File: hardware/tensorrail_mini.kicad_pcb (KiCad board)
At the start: 2 copper layers, 100 x 70 mm, 62 parts, among them J1 USB-C_PWR, J2 JTAG, J3 EXPANSION, SW1 RESET, SW2 BOOT, U1 TPS62130_3V3, U2 TPS62130_1V2, U3 INA219, U4 W25Q128, U5 50MHz

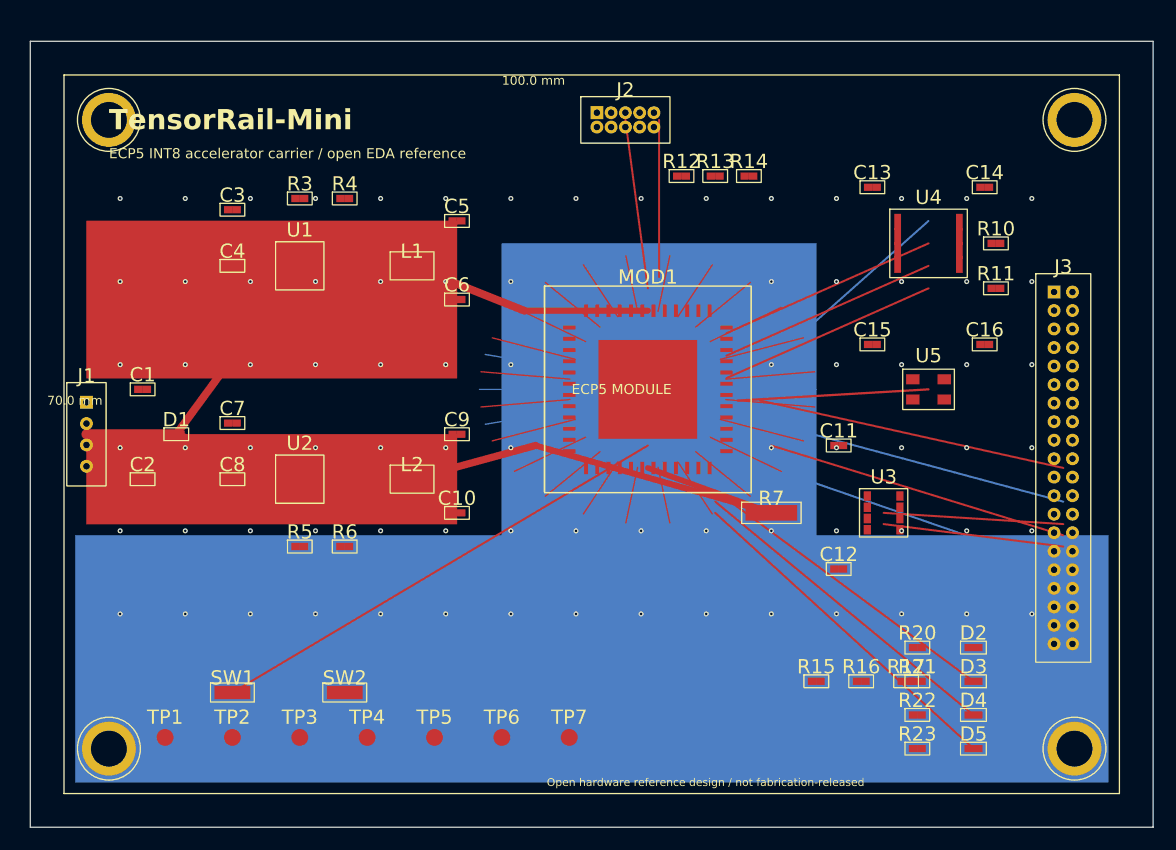
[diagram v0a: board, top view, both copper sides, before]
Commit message: Update TensorRail PCB artifact
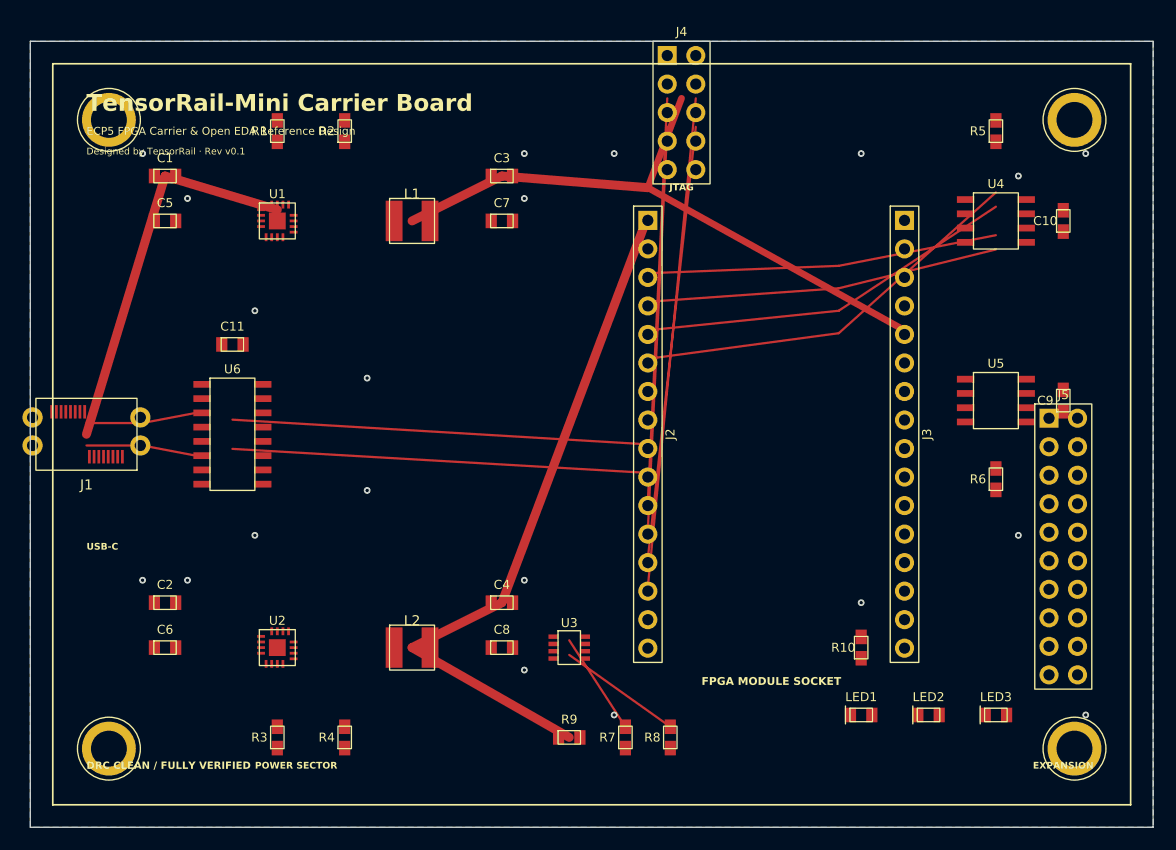
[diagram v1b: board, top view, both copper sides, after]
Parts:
- removed C12: 10n, Discrete_SMD:C12
- removed C13: 100n, Discrete_SMD:C13
- removed C14: 10n, Discrete_SMD:C14
- removed C15: 100n, Discrete_SMD:C15
- removed C16: 10n, Discrete_SMD:C16
- removed D1: PMEG, Discrete_SMD:D1
- removed D2: LED, Discrete_SMD:D2
- removed D3: LED, Discrete_SMD:D3
- removed D4: LED, Discrete_SMD:D4
- removed D5: LED, Discrete_SMD:D5
- removed MOD1: OrangeCrab_85F, Module:ECP5_Feather_Module_Socket
- removed R11: 10k, Discrete_SMD:R11
- removed R12: 100R, Discrete_SMD:R12
- removed R13: 100R, Discrete_SMD:R13
- removed R14: 100R, Discrete_SMD:R14
- removed R15: 4k7, Discrete_SMD:R15
- removed R16: 4k7, Discrete_SMD:R16
- removed R17: 4k7, Discrete_SMD:R17
- removed R20: 330R, Discrete_SMD:R20
- removed R21: 330R, Discrete_SMD:R21
- removed R22: 330R, Discrete_SMD:R22
- removed R23: 330R, Discrete_SMD:R23
- removed SW1: RESET, Discrete_SMD:SW1
- removed SW2: BOOT, Discrete_SMD:SW2
- removed TP1: +5V, TestPoint:TestPoint_Pad_D1.5mm
- removed TP2: +3V3, TestPoint:TestPoint_Pad_D1.5mm
- removed TP3: +1V2, TestPoint:TestPoint_Pad_D1.5mm
- removed TP4: GND, TestPoint:TestPoint_Pad_D1.5mm
- removed TP5: SCL, TestPoint:TestPoint_Pad_D1.5mm
- removed TP6: SDA, TestPoint:TestPoint_Pad_D1.5mm
- removed TP7: CLK_50M, TestPoint:TestPoint_Pad_D1.5mm
- added J4: JTAG, Connector_PinHeader_2.54mm:PinHeader_2x05_P2.54mm_Vertical, F.Cu at (58.0, 6.35)
- added J5: EXPANSION, Connector_PinHeader_2.54mm:PinHeader_2x10_P2.54mm_Vertical, F.Cu at (92.0, 45.0)
- added LED1: Green, LED_SMD:LED_0805_2012Metric, F.Cu at (74.0, 60.0)
- added LED2: Blue, LED_SMD:LED_0805_2012Metric, F.Cu at (80.0, 60.0)
- added LED3: Red, LED_SMD:LED_0805_2012Metric, F.Cu at (86.0, 60.0)
- added R1: 464k, Resistor_SMD:R_0805_2012Metric, F.Cu at (22.0, 8.00)
- added R2: 100k, Resistor_SMD:R_0805_2012Metric, F.Cu at (28.0, 8.00)
- added R8: 10k, Resistor_SMD:R_0805_2012Metric, F.Cu at (57.0, 62.0)
- added R9: 0.1, Resistor_SMD:R_0805_2012Metric, F.Cu at (48.0, 62.0)
- added U6: CH340C, Package_SO:SOIC-16_3.9x9.9mm_P1.27mm, F.Cu at (18.0, 35.0)
- C1: value 100n -> 10u; footprint Discrete_SMD:C1 -> Capacitor_SMD:C_0805_2012Metric
- C10: footprint Discrete_SMD:C10 -> Capacitor_SMD:C_0805_2012Metric
- C11: value 100n -> 22u; footprint Discrete_SMD:C11 -> Capacitor_SMD:C_0805_2012Metric
- C2: value 100n -> 10u; footprint Discrete_SMD:C2 -> Capacitor_SMD:C_0805_2012Metric
- C3: footprint Discrete_SMD:C3 -> Capacitor_SMD:C_0805_2012Metric
- C4: value 100n -> 10u; footprint Discrete_SMD:C4 -> Capacitor_SMD:C_0805_2012Metric
- C5: value 100u -> 100n; footprint Discrete_SMD:C5 -> Capacitor_SMD:C_0805_2012Metric
- C6: footprint Discrete_SMD:C6 -> Capacitor_SMD:C_0805_2012Metric
- C7: value 10u -> 100n; footprint Discrete_SMD:C7 -> Capacitor_SMD:C_0805_2012Metric
- C8: footprint Discrete_SMD:C8 -> Capacitor_SMD:C_0805_2012Metric
- C9: value 100u -> 100n; footprint Discrete_SMD:C9 -> Capacitor_SMD:C_0805_2012Metric
- J1: value USB-C_PWR -> USB-C; footprint Connector_Generic:1x4_Header -> Connector_USB:USB_C_Receptacle_GCT_USB4135
- J2: value JTAG -> Feather Left; footprint Connector_Generic:5x2_Header -> Connector_PinHeader_2.54mm:PinHeader_1x16_P2.54mm_Vertical
- J3: value EXPANSION -> Feather Right; footprint Connector_Generic:2x20_Header -> Connector_PinHeader_2.54mm:PinHeader_1x16_P2.54mm_Vertical
- L1: footprint Discrete_SMD:L1 -> Inductor_SMD:L_Bourns-SRN4018
- L2: footprint Discrete_SMD:L2 -> Inductor_SMD:L_Bourns-SRN4018
- R10: value 10k -> 330; footprint Discrete_SMD:R10 -> Resistor_SMD:R_0805_2012Metric
- R3: value 464k -> 103k; footprint Discrete_SMD:R3 -> Resistor_SMD:R_0805_2012Metric
- R4: footprint Discrete_SMD:R4 -> Resistor_SMD:R_0805_2012Metric
- R5: value 103k -> 10k; footprint Discrete_SMD:R5 -> Resistor_SMD:R_0805_2012Metric
- R6: value 100k -> 10k; footprint Discrete_SMD:R6 -> Resistor_SMD:R_0805_2012Metric
- R7: value 0R1_SHUNT -> 10k; footprint Discrete_SMD:R7 -> Resistor_SMD:R_0805_2012Metric
- U1, U2: footprint Package_TO_SOT_SMD:SOT-23-8 -> Package_DFN_QFN:QFN-16-1EP_3x3mm_P0.5mm_EP1.45x1.45mm
- U5: value 50MHz -> APS6404L-3SQR; footprint Oscillator:Oscillator_3.2x2.5 -> Package_SO:SOIC-8_3.9x4.9mm_P1.27mm
- moved R5 72.2 mm to (86.0, 8.00), turned to 90 degrees
- moved C10 59.9 mm to (92.0, 16.0), turned to 90 degrees
- moved R6 58.3 mm to (86.0, 39.0), turned to 90 degrees
- moved C11 54.7 mm to (18.0, 27.0)
- moved C9 54.1 mm to (92.0, 32.0), turned to 90 degrees
- moved R3 48.0 mm to (22.0, 62.0), turned to 90 degrees
- moved R4 48.0 mm to (28.0, 62.0), turned to 90 degrees
- moved C6 40.5 mm to (12.0, 54.0)
- moved C4 38.4 mm to (42.0, 50.0)
- moved R10 37.9 mm to (74.0, 54.0), turned to 90 degrees
- moved U3 30.5 mm to (48.0, 54.0)
- moved C7 30.0 mm to (42.0, 16.0)
- moved C8 28.3 mm to (42.0, 54.0)
- moved J2 28.1 mm to (55.0, 35.0)
- moved C5 26.0 mm to (12.0, 16.0)
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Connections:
- C1 pad 1: +5V -> VBUS_RAW
- C10 pad 1: +1V2 -> +3V3
- C2 pad 1: +5V -> +3V3
- C3 pad 1: VBUS_RAW -> +3V3
- C4 pad 1: VBUS_RAW -> +1V2
- C5 pad 1: +3V3 -> VBUS_RAW
- C8 pad 1: +3V3 -> +1V2
- C9 pad 1: +1V2 -> +3V3
- J2 pad 10: GND -> UART_TX
- J2 pad 2: JTAG_TDI -> +1V2
- J2 pad 3: RESET_N -> GND
- J2 pad 4: JTAG_TDO -> SPI_SCK
- J2 pad 5: JTAG_TCK -> SPI_MOSI
- J2 pad 6: RESET_N -> SPI_MISO
- J2 pad 7: JTAG_TMS -> SPI_CS_FLASH
- J2 pad 8: (no net) -> CLK_50M
- J2 pad 9: GND -> RESET_N
- J3 pad 1: +3V3 -> GPIO1
- J3 pad 10: SDA -> SPI_MOSI
- J3 pad 11: SPI_SCK -> SPI_MISO
- J3 pad 12: SPI_MOSI -> SPI_CS_FLASH
- J3 pad 13: SPI_MISO -> CLK_50M
- J3 pad 14: SPI_CS_FLASH -> RESET_N
- J3 pad 15: RESET_N -> UART_TX
- J3 pad 16: BOOT_N -> UART_RX
- J3 pad 2: GND -> GPIO2
- J3 pad 3: GPIO0 -> GPIO3
- J3 pad 4: GPIO1 -> PSRAM0
- J3 pad 5: GPIO2 -> PSRAM1
- J3 pad 6: GPIO3 -> +3V3
- J3 pad 7: UART_TX -> +1V2
- J3 pad 8: UART_RX -> GND
- J3 pad 9: SCL -> SPI_SCK
- R10 pad 2: SPI_CS_FLASH -> LED_DONE
- R3 pad 1: +3V3 -> +1V2
- R3 pad 2: FB_3V3 -> FB_1V2
- R4 pad 1: FB_3V3 -> FB_1V2
- R5 pad 1: +1V2 -> +3V3
- R5 pad 2: FB_1V2 -> SPI_CS_FLASH
- R6 pad 1: FB_1V2 -> +3V3
- R6 pad 2: GND -> PSRAM0
- R7 pad 1: +1V2 -> +3V3
- R7 pad 2: VCORE_SENSED -> SCL
- U1 pad 3: FB_3V3 -> VBUS_RAW
- U1 pad 4: (no net) -> GND
- U1 pad 5: GND -> +3V3
- U1 pad 6: SW_3V3 -> FB_3V3
- U1 pad 7: (no net) -> GND
- U1 pad 8: +3V3 -> GND
- U2 pad 3: FB_1V2 -> +3V3
- U2 pad 4: (no net) -> GND
- U2 pad 5: GND -> +1V2
- U2 pad 6: SW_1V2 -> FB_1V2
- U2 pad 7: (no net) -> GND
- U2 pad 8: +1V2 -> GND
- U3 pad 8: +3V3 -> GND
- U5 pad 1: GND -> PSRAM0
- U5 pad 2: GND -> PSRAM1
- U5 pad 3: CLK_50M -> +3V3
- U5 pad 4: +3V3 -> GND
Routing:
- net GPIO0: track 67.2 -> 10.3 mm
- net GPIO1: track 66.5 -> 10.3 mm
- net JTAG_TDO: track 0.00 -> 43.7 mm
- net RESET_N: track 43.0 -> 0.00 mm
- net GND: track 39.6 -> 0.00 mm, vias 81 -> 20
- net JTAG_TDI: track 0.00 -> 38.7 mm
- net BOOT_N: track 35.0 -> 0.00 mm
- net LED_HB: track 31.1 -> 0.00 mm
- net LED_DONE: track 29.8 -> 0.00 mm
- net LED_BUSY: track 28.6 -> 0.00 mm
- net SPI_SCK: track 59.2 -> 31.3 mm
- net SPI_MOSI: track 59.2 -> 31.5 mm
- net SPI_MISO: track 59.2 -> 33.9 mm
- net JTAG_TMS: track 14.0 -> 35.9 mm
- net JTAG_TCK: track 15.1 -> 35.9 mm
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- added copper zone on B.Cu, net GND
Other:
- board text added: "DRC CLEAN / FULLY VERIFIED"
- board text added: "Designed by TensorRail · Rev v0.1"
- board text added: "ECP5 FPGA Carrier & Open EDA Reference Design"
- board text added: "EXPANSION"
- board text added: "FPGA MODULE SOCKET"
- board text added: "JTAG"
- board text added: "POWER SECTOR"
- board text added: "TensorRail-Mini Carrier Board"
- board text added: "USB-C"
- board text removed: "100.0 mm"
- board text removed: "70.0 mm"
- board text removed: "ECP5 INT8 accelerator carrier / open EDA reference"
- board text removed: "Open hardware reference design / not fabrication-released"
- board text removed: "TensorRail-Mini"
